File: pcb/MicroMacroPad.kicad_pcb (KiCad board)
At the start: 2 copper layers, 63.5 x 99.9 mm, 39 parts, among them J1 Conn_01x04_Pin, SW1 SW_Push, SW10 SW_Push, SW11 SW_Push, SW12 SW_Push, SW2 SW_Push, SW3 SW_Push, SW4 SW_Push, SW5 SW_Push, SW6 SW_Push, SW7 SW_Push, SW8 SW_Push, SW9 SW_Push, U1 XIAO-RP2040-DIP

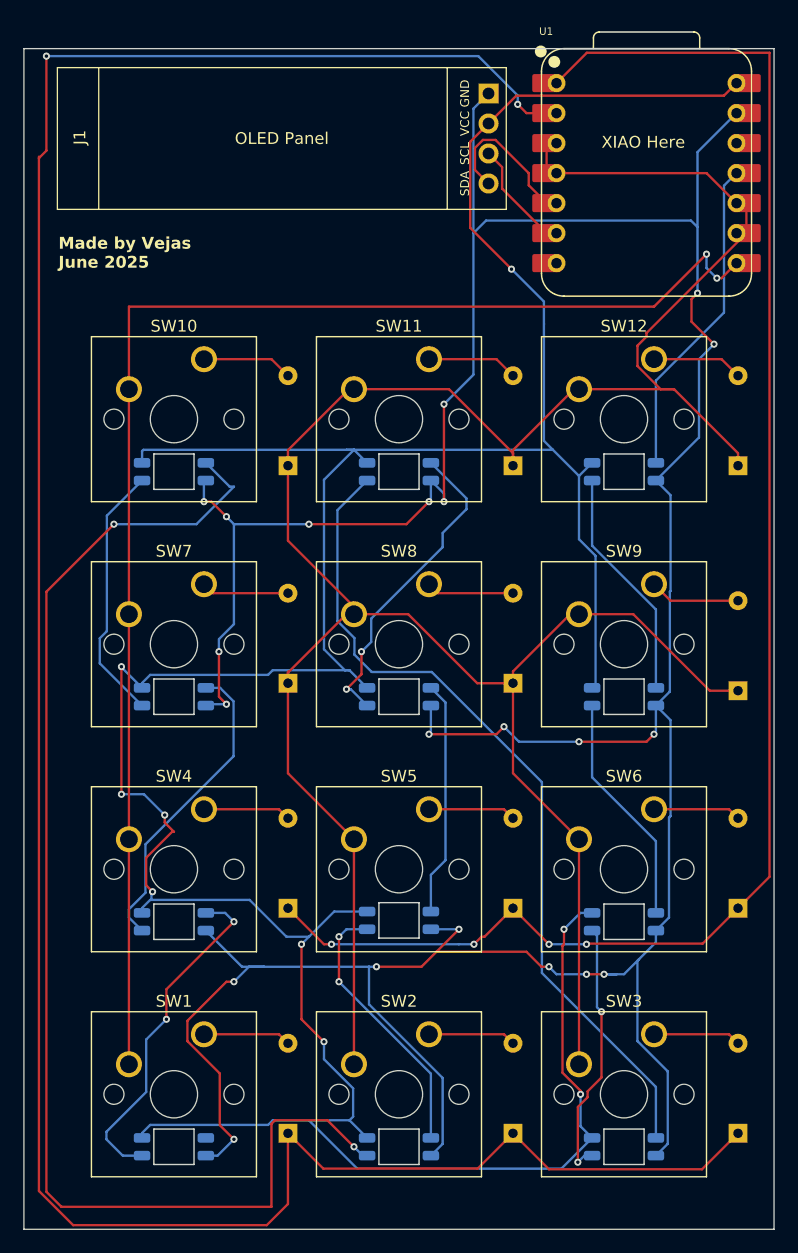
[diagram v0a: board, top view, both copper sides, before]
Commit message: V2 upload
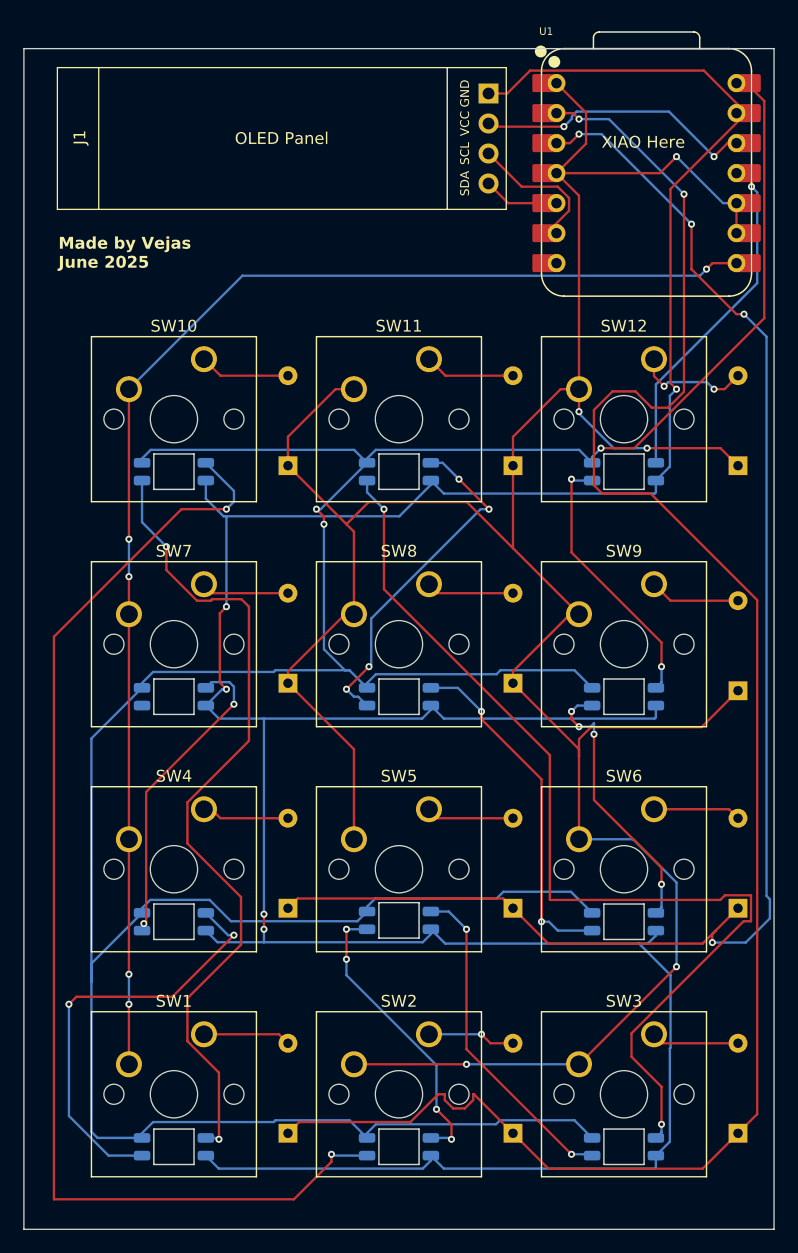
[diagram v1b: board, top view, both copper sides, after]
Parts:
- J1: footprint kicad-footprint:SSD1306-0.91-OLED-4pin-128x32 -> footprints:SSD1306-0.91-OLED-4pin-128x32
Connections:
- D1 pad 1: col2 -> row2
- D10 pad 1: col0 -> col2
- D11 pad 1: col0 -> col2
- D12 pad 1: col0 -> col2
- D16 pad 2: Net-(D15-DOUT) -> Net-(D16-DOUT)
- D18 pad 4: Net-(D18-DIN) -> Net-(D15-DOUT)
- D19 pad 4: Net-(D18-DIN) -> Net-(D16-DOUT)
- D2 pad 1: col2 -> row2
- D22 pad 2: Net-(D21-DOUT) -> unconnected-(D22-DOUT-Pad2)
- D24 pad 4: unconnected-(D24-DIN-Pad4) -> Net-(D21-DOUT)
- D3 pad 1: col2 -> row2
- D4 pad 1: col1 -> row3
- D5 pad 1: col1 -> row3
- D6 pad 1: col1 -> row3
- D7 pad 1: col0 -> col2
- D8 pad 1: col0 -> col2
- D9 pad 1: col0 -> col2
- J1 pad 2: +5V -> +3V3
- SW1 pad 2: row0 -> col1
- SW10 pad 2: row0 -> col1
- SW11 pad 2: col0 -> col2
- SW12 pad 2: col0 -> col2
- SW2 pad 2: col0 -> col2
- SW3 pad 2: col0 -> col2
- SW4 pad 2: row0 -> col1
- SW5 pad 2: col0 -> col2
- SW6 pad 2: col0 -> col2
- SW7 pad 2: row0 -> col1
- SW8 pad 2: col0 -> col2
- SW9 pad 2: col0 -> col2
- U1 pad 1: col1 -> col2
- U1 pad 10: col0 -> col2
- U1 pad 12: unconnected-(U1-3V3-Pad12) -> +3V3
- U1 pad 2: col2 -> row2
- U1 pad 3: col0 -> row3
- U1 pad 4: col0 -> col2
- U1 pad 8: row0 -> col1
- U1 pad 9: col0 -> col2
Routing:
- net col0: track 226.1 -> 0.00 mm
- net row2: track 0.00 -> 155.5 mm, vias 0 -> 2
- net row3: track 0.00 -> 125.7 mm, vias 0 -> 4
- net row0: track 119.5 -> 0.00 mm, vias 2 -> 0
- net Net-(D21-DOUT): track 22.0 -> 70.1 mm, vias 0 -> 2
- net col2: track 213.4 -> 244.3 mm, vias 2 -> 5
- net GND: track 310.2 -> 279.8 mm, vias 21 -> 5
- net Net-(D16-DOUT): track 0.00 -> 28.2 mm, vias 0 -> 2
- net +3V3: track 0.00 -> 24.6 mm, vias 0 -> 2
- net col1: track 135.8 -> 113.8 mm, vias 4 -> 5
- net Net-(D18-DIN): track 20.0 -> 0.00 mm
- net Net-(D16-DIN): track 70.8 -> 85.4 mm, vias 0 -> 2
- net +5V: track 291.5 -> 276.9 mm, vias 9 -> 3
- net Net-(D20-DOUT): track 109.6 -> 100.4 mm
- net Net-(D23-DIN): track 29.2 -> 36.6 mm
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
